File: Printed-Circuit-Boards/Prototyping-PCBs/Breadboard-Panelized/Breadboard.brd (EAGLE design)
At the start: 91.4 x 96.5 mm, 196 parts

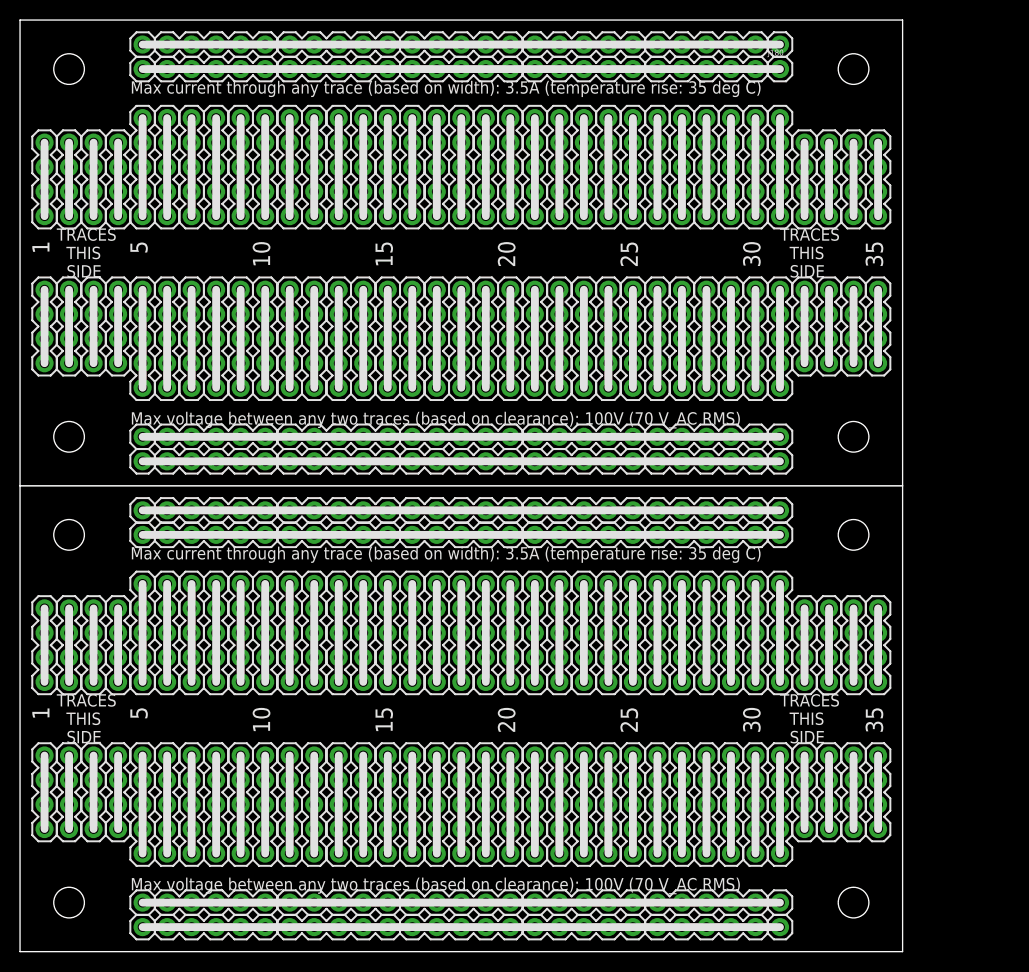
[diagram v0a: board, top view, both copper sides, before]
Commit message: Updated PCB files.
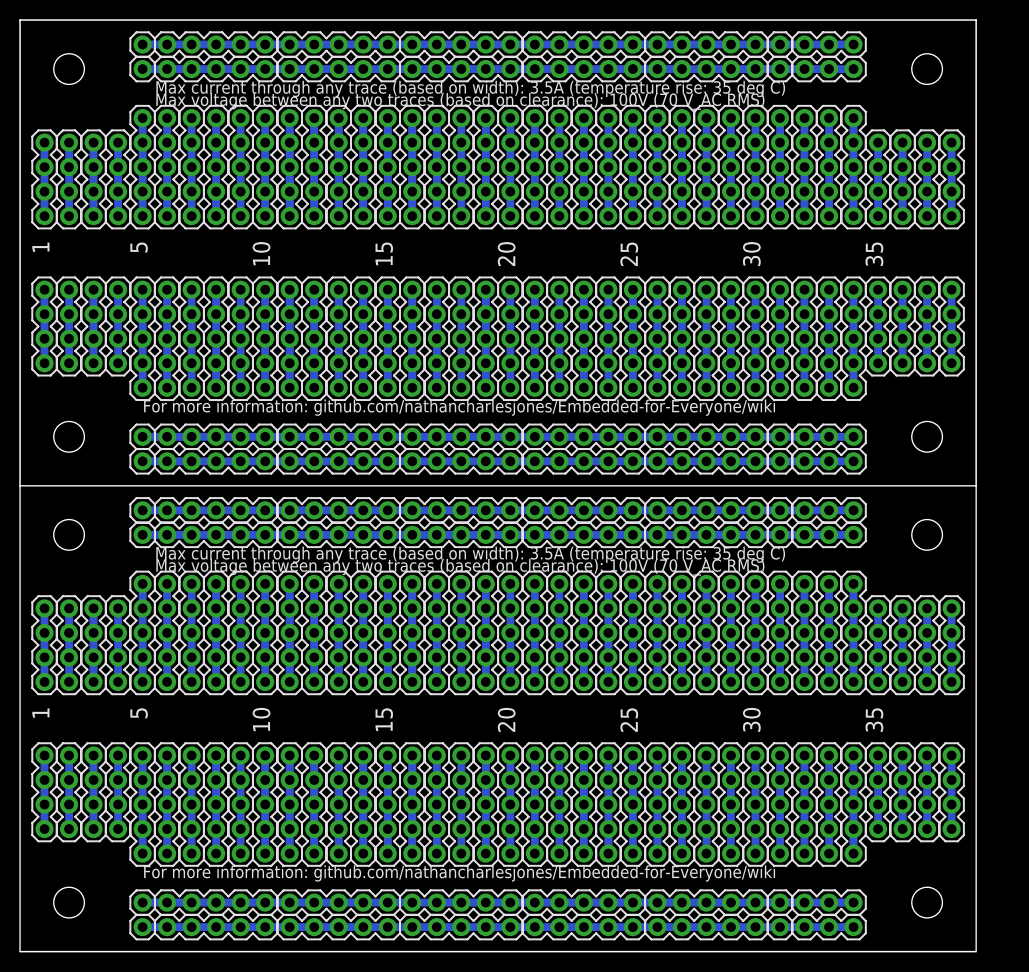
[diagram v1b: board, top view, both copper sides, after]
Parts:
- added J197, J198, J199, J200, J203, J204, J205, J206: (no value), SparkFun-Connectors:1X04
- added J201, J202: (no value), SparkFun-Connectors:1X01
- added J207, J208, J209, J210, J211, J212: (no value), SparkFun-Connectors:1X05
- added J213, J214, J215, J216: 455-1750-1-ND, SparkFun-Connectors:1X03
- J173, J174, J179, J180: device SparkFun-Connectors:1X01 -> SparkFun-Connectors:1X05
- J175, J176, J177, J178, J181, J182: device SparkFun-Connectors:1X04 -> SparkFun-Connectors:1X05
- J183, J184, J189, J190, J195, J196: device SparkFun-Connectors:1X04 -> SparkFun-Connectors:1X01
- J185, J186, J191, J192: device SparkFun-Connectors:1X01 -> SparkFun-Connectors:1X04
- J51, J52, J53, J54: value (none) -> 455-1750-1-ND; device SparkFun-Connectors:1X05 -> SparkFun-Connectors:1X03
- moved J45 106.7 mm to (81.3, 10.2), turned to 90 degrees
- moved J51 101.5 mm to (81.3, 5.08)
- moved J46 100.7 mm to (83.8, 10.2), turned to 90 degrees
- moved J52 97.7 mm to (81.3, 2.54)
- moved J47 95.5 mm to (86.4, 10.2), turned to 90 degrees
- moved J50 95.3 mm to (86.4, 27.9), turned to 90 degrees
- moved J187 92.7 mm to (94.0, 76.2)
- moved J188 92.7 mm to (96.5, 76.2)
- moved J193 92.7 mm to (94.0, 61.0)
- moved J194 92.7 mm to (96.5, 61.0)
- moved J192 84.4 mm to (91.4, 61.0), turned to 90 degrees
- moved J191 83.0 mm to (88.9, 61.0), turned to 90 degrees
- moved J186 82.7 mm to (91.4, 76.2), turned to 90 degrees
- moved J185 79.6 mm to (88.9, 76.2), turned to 90 degrees
- moved J189 71.8 mm to (78.7, 50.8), turned to 0 degrees
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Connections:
- removed net N$110 (its old number): J181.1, J181.2, J181.3, J181.4
- removed net N$111 (its old number): J182.1, J182.2, J182.3, J182.4
- removed net N$112 (its old number): J183.1, J183.2, J183.3, J183.4
- removed net N$113 (its old number): J184.1, J184.2, J184.3, J184.4
- removed net N$89 (its old number): J125.1, J125.2, J125.3, J125.4, J125.5
- removed net N$90 (its old number): J126.1, J126.2, J126.3, J126.4, J126.5
- removed net N$91 (its old number): J127.1, J127.2, J127.3, J127.4, J127.5
- removed net N$92 (its old number): J128.1, J128.2, J128.3, J128.4, J128.5
- new net N$120: J197.1, J197.2, J197.3, J197.4
- new net N$121: J198.1, J198.2, J198.3, J198.4
- new net N$122: J199.1, J199.2, J199.3, J199.4
- new net N$123: J200.1, J200.2, J200.3, J200.4
- new net N$141: J173.1, J173.2, J173.3, J173.4, J173.5
- new net N$142: J174.1, J174.2, J174.3, J174.4, J174.5
- new net N$143: J175.1, J175.2, J175.3, J175.4, J175.5
- new net N$144: J176.1, J176.2, J176.3, J176.4, J176.5
- new net N$149: J181.1, J181.2, J181.3, J181.4, J181.5
- new net N$150: J182.1, J182.2, J182.3, J182.4, J182.5
- new net N$151: J185.1, J185.2, J185.3, J185.4
- new net N$152: J186.1, J186.2, J186.3, J186.4
- new net N$155: J207.1, J207.2, J207.3, J207.4, J207.5
- new net N$156: J208.1, J208.2, J208.3, J208.4, J208.5
- new net N$157: J209.1, J209.2, J209.3, J209.4, J209.5
- new net N$158: J210.1, J210.2, J210.3, J210.4, J210.5
- new net N$159: J211.1, J211.2, J211.3, J211.4, J211.5
- new net N$160: J212.1, J212.2, J212.3, J212.4, J212.5
- new net N$79: J49.1, J49.2, J49.3, J49.4, J49.5
- new net N$80: J50.1, J50.2, J50.3, J50.4, J50.5
- net N$1: now also J52.1, J52.2, J52.3
- net N$116: now also J191.1, J191.2, J191.3, J191.4; no longer J189.1, J189.2, J189.3, J189.4
- net N$117: now also J192.1, J192.2, J192.3, J192.4; no longer J190.1, J190.2, J190.3, J190.4
- net N$145: now also J177.1, J177.2, J177.3, J177.4, J177.5; no longer J175.1, J175.2, J175.3, J175.4
- net N$146: now also J178.1, J178.2, J178.3, J178.4, J178.5; no longer J176.1, J176.2, J176.3, J176.4
- net N$147: now also J179.1, J179.2, J179.3, J179.4, J179.5; no longer J177.1, J177.2, J177.3, J177.4
- net N$148: now also J180.1, J180.2, J180.3, J180.4, J180.5; no longer J178.1, J178.2, J178.3, J178.4
- net N$2: now also J51.1, J51.2, J51.3
- net N$3: now also J54.1, J54.2, J54.3
- net N$4: now also J53.1, J53.2, J53.3
- net N$75: no longer J179.1, J191.1, J45.1, J45.2, J45.3, J45.4, J45.5, J46.1, J46.2, J46.3, J46.4, J46.5, J47.1, J47.2, J47.3, J47.4, J47.5, J49.1, J49.2, J49.3, J49.4, J49.5
- net N$76: now also J45.1, J45.2, J45.3, J45.4, J45.5; no longer J180.1, J192.1, J50.1, J50.2, J50.3, J50.4, J50.5, J51.1, J51.2, J51.3, J51.4, J51.5, J52.1, J52.2, J52.3, J52.4, J52.5, J53.1, J53.2, J53.3, J53.4, J53.5, J54.1, J54.2, J54.3, J54.4, J54.5
- net N$77: now also J46.1, J46.2, J46.3, J46.4, J46.5; no longer J173.1, J185.1, J55.1, J55.2, J55.3, J55.4, J55.5, J56.1, J56.2, J56.3, J56.4, J56.5, J57.1, J57.2, J57.3, J57.4, J57.5, J58.1, J58.2, J58.3, J58.4, J58.5, J59.1, J59.2, J59.3, J59.4, J59.5
- net N$78: now also J47.1, J47.2, J47.3, J47.4, J47.5; no longer J174.1, J186.1, J60.1, J60.2, J60.3, J60.4, J60.5, J88.1, J88.2, J88.3, J88.4, J88.5, J89.1, J89.2, J89.3, J89.4, J89.5, J90.1, J90.2, J90.3, J90.4, J90.5, J91.1, J91.2, J91.3, J91.4, J91.5
- net N$81: now also J189.1, J201.1, J214.1, J214.2, J214.3, J55.1, J55.2, J55.3, J55.4, J55.5, J56.1, J56.2, J56.3, J56.4, J56.5, J57.1, J57.2, J57.3, J57.4, J57.5, J58.1, J58.2, J58.3, J58.4, J58.5, J59.1, J59.2, J59.3, J59.4, J59.5; no longer J195.1, J195.2, J195.3, J195.4
- net N$82: now also J190.1, J202.1, J213.1, J213.2, J213.3, J60.1, J60.2, J60.3, J60.4, J60.5, J88.1, J88.2, J88.3, J88.4, J88.5, J89.1, J89.2, J89.3, J89.4, J89.5, J90.1, J90.2, J90.3, J90.4, J90.5, J91.1, J91.2, J91.3, J91.4, J91.5; no longer J196.1, J196.2, J196.3, J196.4
- net N$83: now also J123.1, J123.2, J123.3, J123.4, J123.5, J183.1, J195.1, J216.1, J216.2, J216.3, J93.1, J93.2, J93.3, J93.4, J93.5, J94.1, J94.2, J94.3, J94.4, J94.5, J95.1, J95.2, J95.3, J95.4, J95.5
- net N$84: now also J124.1, J124.2, J124.3, J124.4, J124.5, J125.1, J125.2, J125.3, J125.4, J125.5, J126.1, J126.2, J126.3, J126.4, J126.5, J127.1, J127.2, J127.3, J127.4, J127.5, J128.1, J128.2, J128.3, J128.4, J128.5, J184.1, J196.1, J215.1, J215.2, J215.3; no longer J93.1, J93.2, J93.3, J93.4, J93.5
- net N$85: now also J203.1, J203.2, J203.3, J203.4; no longer J94.1, J94.2, J94.3, J94.4, J94.5
- net N$86: now also J204.1, J204.2, J204.3, J204.4; no longer J95.1, J95.2, J95.3, J95.4, J95.5
- net N$87: now also J205.1, J205.2, J205.3, J205.4; no longer J123.1, J123.2, J123.3, J123.4, J123.5
- net N$88: now also J206.1, J206.2, J206.3, J206.4; no longer J124.1, J124.2, J124.3, J124.4, J124.5
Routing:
- net N$82: track 7.62 -> 73.7 mm
- net N$81: track 7.62 -> 73.7 mm
- net N$84: track 10.2 -> 73.7 mm
- net N$83: track 10.2 -> 73.7 mm
- net N$78: track 66.0 -> 10.2 mm
- net N$77: track 66.0 -> 10.2 mm
- net N$76: track 66.0 -> 10.2 mm
- net N$75: track 66.0 -> 10.2 mm
- net N$80: track 0.00 -> 10.2 mm
- net N$79: track 0.00 -> 10.2 mm
- net N$92 (its old number): track 10.2 -> 0.00 mm
- net N$91 (its old number): track 10.2 -> 0.00 mm
- net N$90 (its old number): track 10.2 -> 0.00 mm
- net N$89 (its old number): track 10.2 -> 0.00 mm
- net N$160: track 0.00 -> 10.2 mm
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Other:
- board size 91.4 x 96.5 mm -> 99.1 x 96.5 mm
- board text added: "For more information: github.com/nathancharlesjones/Embedded-for-Everyone/wiki"
- board text removed: "For more information: https://github.com/nathancharlesjones/Embedded-for-Everyone"
